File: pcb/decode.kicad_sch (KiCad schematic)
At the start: 22 parts, among them Q1104 2N7002a, Q83 2N7002a, Q84 2N7002a, Q85 2N7002a, Q86 2N7002a, Q87 2N7002a, Q88 2N7002a, Q89 2N7002a, Q90 2N7002a, Q91 2N7002a, Q92 2N7002a, Q93 2N7002a, Q94 2N7002a, Q95 2N7002a, Q96 2N7002a

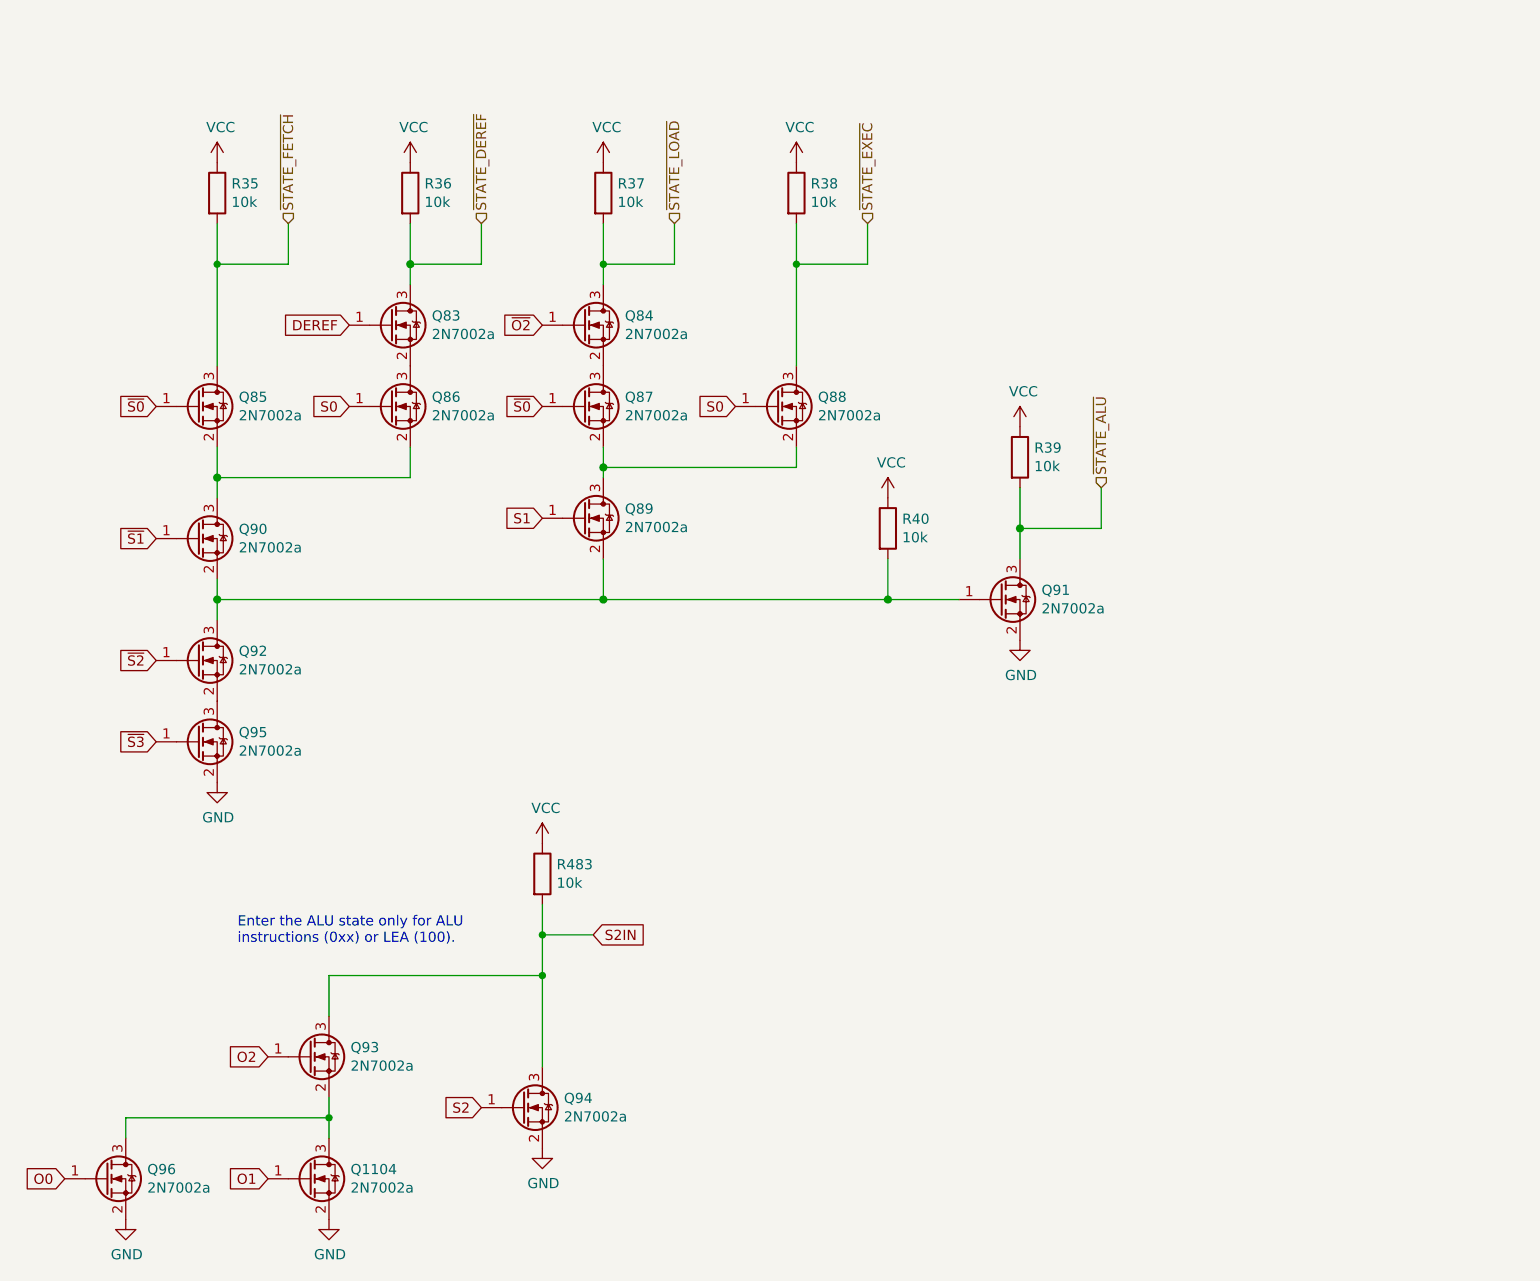
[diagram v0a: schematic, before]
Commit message: Some fixes.
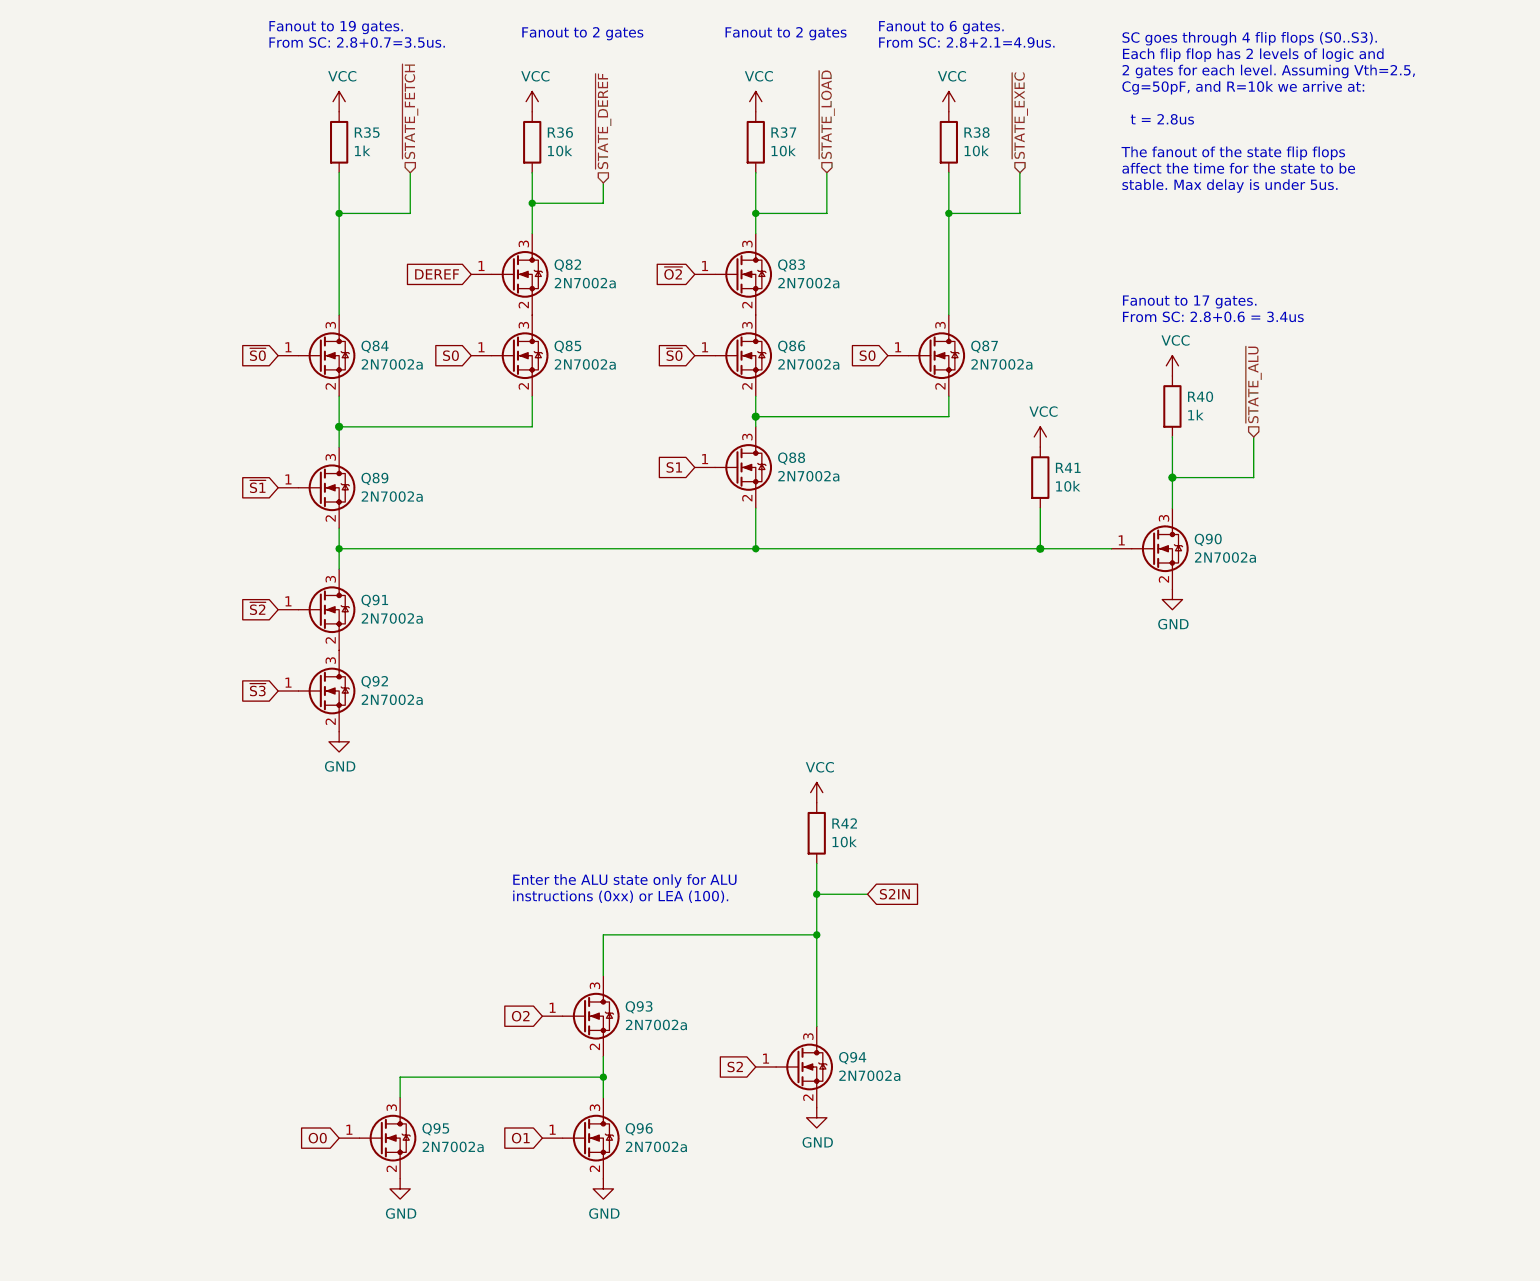
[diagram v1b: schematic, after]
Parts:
- removed R39: 10k, Resistor_SMD:R_0805_2012Metric, symbol Device:R
- added R40: 1k, Resistor_SMD:R_0805_2012Metric, symbol Device:R
- R35: value 10k -> 1k; LCSC C17414 -> C17513
- renumbered Q83 to Q82, Q84 to Q83, Q85 to Q84, Q86 to Q85, Q87 to Q86, Q88 to Q87, Q89 to Q88, Q90 to Q89, Q91 to Q90, Q92 to Q91, Q95 to Q92, Q96 to Q95, Q1104 to Q96, R40 to R41, R483 to R42
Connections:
- net VCC: now also R40.1
- net ~STATE_ALU: now also R40.2
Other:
- note added: "Fanout to 17 gates. From SC: 2.8+0.6 = 3.4us"
- note added: "Fanout to 19 gates. From SC: 2.8+0.7=3.5us."
- note added: "Fanout to 2 gates"
- note added: "Fanout to 6 gates. From SC: 2.8+2.1=4.9us."
- note added: "SC goes through 4 flip flops (S0..S3). Each flip flop has 2 levels of logic and 2 gates for each level. Assuming Vth=2.5, Cg=50pF, and R=10k we arrive at: t = 2.8us The fanout of the state flip flops affect the time for the state to be stable. Max delay is under 5us."
- moved on the sheet: Q82, Q83, Q84, Q85, Q86, Q87, Q88, Q89, Q90, Q91, Q92, Q93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
